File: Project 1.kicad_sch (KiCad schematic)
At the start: 14 parts, among them J1 DB9_Female, J2 Barrel_Jack, P1 RFID-RC522-MODULE, SW1 SW_DPDT_x2, U1 PIC16F1512-ISP, U2 PIC16F1512-ISP, U3 PIC16F1512-ISP, U4 ADG419BN, U5 TM1637, U6 TM1637

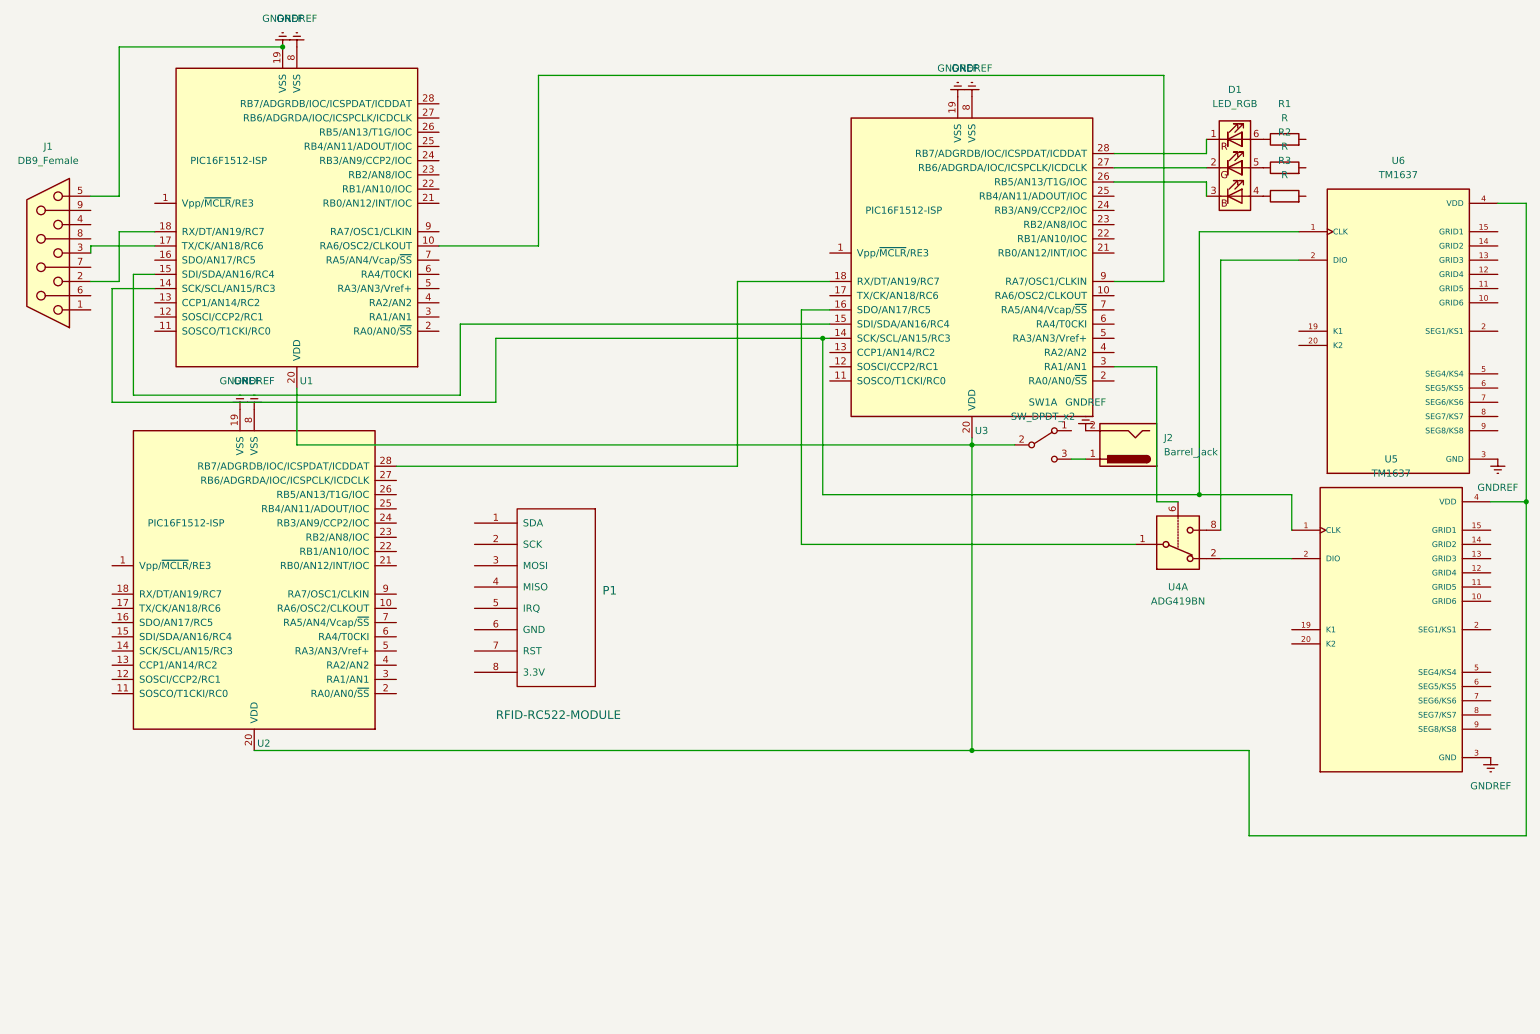
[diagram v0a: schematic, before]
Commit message: Nieuwe tekening begin nieuw schema
Nieuwe tekening begin nieuw schema
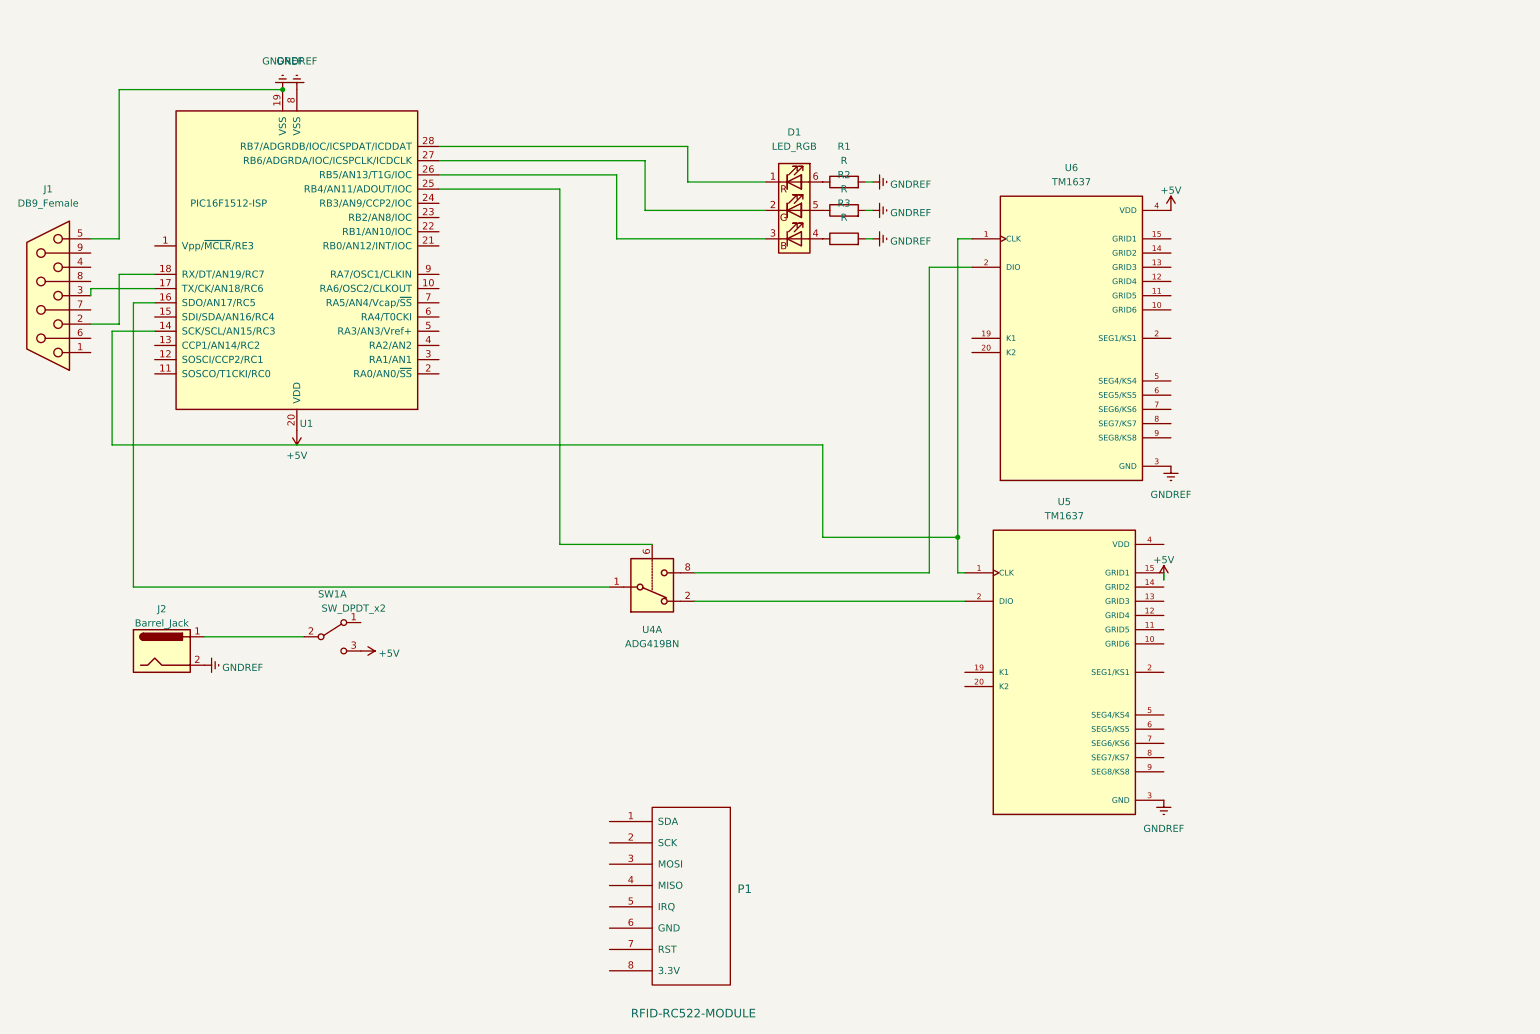
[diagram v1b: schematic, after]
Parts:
- removed U2: PIC16F1512-ISP, Package_DIP:DIP-28_W7.62mm, symbol MCU_Microchip_PIC16:PIC16F1512-ISP
- removed U3: PIC16F1512-ISP, Package_DIP:DIP-28_W7.62mm_Socket, symbol MCU_Microchip_PIC16:PIC16F1512-ISP
- D1: footprint (none) -> LED_SMD:LED_Avago_PLCC6_3x2.8mm
- R1, R2, R3: footprint (none) -> Resistor_SMD:R_0201_0603Metric
- SW1: footprint (none) -> Button_Switch_THT:SW_CuK_JS202011AQN_DPDT_Angled
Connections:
- net GNDREF: now also R1.2, R2.2, R3.2
- net at U6.2 (SEG1/KS1): now also U4.8
- net +5V: now reaches U1.20 (VDD), U6.4 (VDD)
- net +5V: now also SW1.3 (C), U5.15 (GRID1); no longer SW1.2 (B), U5.4 (VDD)
- net at D1.1 (RK): now also U1.28 (RB7/ADGRDB/IOC/ICSPDAT/ICDDAT)
- net at D1.2 (GK): now also U1.27 (RB6/ADGRDA/IOC/ICSPCLK/ICDCLK)
- net at D1.3 (BK): now also U1.26 (RB5/AN13/T1G/IOC)
- net at U5.2 (SEG1/KS1): now also U4.2
- net at J2.1: now also SW1.2 (B); no longer SW1.3 (C)
- net at U4.1: now also U1.16 (SDO/AN17/RC5)
- net at U4.6: now also U1.25 (RB4/AN11/ADOUT/IOC)
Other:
- moved on the sheet: D1, J1, J2, P1, R1, R2, R3, SW1A, U1, U4A, U5, U6

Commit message: ZElfde
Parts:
- P1: footprint Connector_PinHeader_1.27mm:PinHeader_1x08_P1.27mm_Vertical -> Connector_PinSocket_2.54mm:PinSocket_1x08_P2.54mm_Vertical
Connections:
- net at U6.2 (SEG1/KS1): now also U4.8
- net at U5.2 (SEG1/KS1): now also U4.2
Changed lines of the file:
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@@
   (symbol (lib_id "power:+5V") (at 218.44 105.41 0) (unit 1)
     (in_bom yes) (on_board yes) (fields_autoplaced)
-    (property "Reference" "#PWR?" (id 0) (at 218.44 109.22 0)
+    (property "Reference" "#PWR0112" (id 0) (at 218.44 109.22 0)
       (effects (font (size 1.27 1.27)) hide)
     )
@@
   (symbol (lib_id "power:+5V") (at 74.93 118.11 270) (unit 1)
     (in_bom yes) (on_board yes) (fields_autoplaced)
-    (property "Reference" "#PWR?" (id 0) (at 71.12 118.11 0)
+    (property "Reference" "#PWR0104" (id 0) (at 71.12 118.11 0)
       (effects (font (size 1.27 1.27)) hide)
     )
@@
   (symbol (lib_id "power:GNDREF") (at 166.37 34.29 90) (unit 1)
     (in_bom yes) (on_board yes)
-    (property "Reference" "#PWR?" (id 0) (at 172.72 34.29 0)
+    (property "Reference" "#PWR0106" (id 0) (at 172.72 34.29 0)
       (effects (font (size 1.27 1.27)) hide)
     )
@@
   (symbol (lib_id "power:+5V") (at 63.5 78.74 180) (unit 1)
     (in_bom yes) (on_board yes) (fields_autoplaced)
-    (property "Reference" "#PWR?" (id 0) (at 63.5 74.93 0)
+    (property "Reference" "#PWR0105" (id 0) (at 63.5 74.93 0)
       (effects (font (size 1.27 1.27)) hide)
     )
@@
       (effects (font (size 1.524 1.524)) (justify left))
     )
-    (property "Footprint" "Connector_PinHeader_1.27mm:PinHeader_1x08_P1.27mm_Vertical" (id 2) (at 133.35 162.56 0)
+    (property "Footprint" "Connector_PinSocket_2.54mm:PinSocket_1x08_P2.54mm_Vertical" (id 2) (at 133.35 162.56 0)
       (effects (font (size 1.524 1.524)) hide)
     )
@@
   (symbol (lib_id "power:GNDREF") (at 46.99 120.65 90) (unit 1)
     (in_bom yes) (on_board yes) (fields_autoplaced)
-    (property "Reference" "#PWR?" (id 0) (at 53.34 120.65 0)
+    (property "Reference" "#PWR0101" (id 0) (at 53.34 120.65 0)
       (effects (font (size 1.27 1.27)) hide)
     )
@@
   (symbol (lib_id "power:GNDREF") (at 166.37 44.45 90) (unit 1)
     (in_bom yes) (on_board yes) (fields_autoplaced)
-    (property "Reference" "#PWR?" (id 0) (at 172.72 44.45 0)
+    (property "Reference" "#PWR0107" (id 0) (at 172.72 44.45 0)
       (effects (font (size 1.27 1.27)) hide)
     )
@@
   (symbol (lib_id "power:+5V") (at 219.71 39.37 0) (unit 1)
     (in_bom yes) (on_board yes)
-    (property "Reference" "#PWR?" (id 0) (at 219.71 43.18 0)
+    (property "Reference" "#PWR0111" (id 0) (at 219.71 43.18 0)
       (effects (font (size 1.27 1.27)) hide)
     )
@@
   (symbol (lib_id "power:GNDREF") (at 166.37 39.37 90) (unit 1)
     (in_bom yes) (on_board yes)
-    (property "Reference" "#PWR?" (id 0) (at 172.72 39.37 0)
+    (property "Reference" "#PWR0110" (id 0) (at 172.72 39.37 0)
       (effects (font (size 1.27 1.27)) hide)
     )
@@
   )
   (symbol_instances
+    (path "/ba3feac5-d630-4bed-8e14-7db0b42c2f83"
+      (reference "#PWR0101") (unit 1) (value "GNDREF") (footprint "")
+    )
     (path "/c7669069-c13b-42b4-a278-9f48cd76a941"
       (reference "#PWR0102") (unit 1) (value "GNDREF") (footprint "")
@@
       (reference "#PWR0103") (unit 1) (value "GNDREF") (footprint "")
     )
+    (path "/338518ab-5898-4c83-bb50-b440f75027b4"
+      (reference "#PWR0104") (unit 1) (value "+5V") (footprint "")
+    )
+    (path "/78869d40-832b-4402-9c11-4193141d6842"
+      (reference "#PWR0105") (unit 1) (value "+5V") (footprint "")
+    )
+    (path "/6a39bd7f-5728-47af-939f-6a17becf1f25"
+      (reference "#PWR0106") (unit 1) (value "GNDREF") (footprint "")
+    )
+    (path "/cb63e662-501d-4536-84b1-4962a1f99666"
+      (reference "#PWR0107") (unit 1) (value "GNDREF") (footprint "")
+    )
     (path "/d88cfbbf-1cde-4824-a59d-8811cec5ba8c"
       (reference "#PWR0108") (unit 1) (value "GNDREF") (footprint "")
@@
       (reference "#PWR0109") (unit 1) (value "GNDREF") (footprint "")
     )
+    (path "/f606cdc7-a5e0-4feb-bca6-f9655c59631f"
+      (reference "#PWR0110") (unit 1) (value "GNDREF") (footprint "")
+    )
+    (path "/ce0fc0c8-3db8-4941-80cc-972bfb47b4fe"
+      (reference "#PWR0111") (unit 1) (value "+5V") (footprint "")
+    )
     (path "/0a625eb3-7c7b-4204-8a93-2f92b04ba9f2"
-      (reference "#PWR?") (unit 1) (value "+5V") (footprint "")
-    )
-    (path "/338518ab-5898-4c83-bb50-b440f75027b4"
-      (reference "#PWR?") (unit 1) (value "+5V") (footprint "")
-    )
-    (path "/6a39bd7f-5728-47af-939f-6a17becf1f25"
-      (reference "#PWR?") (unit 1) (value "GNDREF") (footprint "")
-    )
-    (path "/78869d40-832b-4402-9c11-4193141d6842"
-      (reference "#PWR?") (unit 1) (value "+5V") (footprint "")
-    )
-    (path "/ba3feac5-d630-4bed-8e14-7db0b42c2f83"
-      (reference "#PWR?") (unit 1) (value "GNDREF") (footprint "")
-    )
-    (path "/cb63e662-501d-4536-84b1-4962a1f99666"
-      (reference "#PWR?") (unit 1) (value "GNDREF") (footprint "")
-    )
-    (path "/ce0fc0c8-3db8-4941-80cc-972bfb47b4fe"
-      (reference "#PWR?") (unit 1) (value "+5V") (footprint "")
-    )
-    (path "/f606cdc7-a5e0-4feb-bca6-f9655c59631f"
-      (reference "#PWR?") (unit 1) (value "GNDREF") (footprint "")
+      (reference "#PWR0112") (unit 1) (value "+5V") (footprint "")
     )
     (path "/2de269c6-be7f-498e-9d9c-81e85907e612"
@@
     )
     (path "/a96f00ba-dda0-463c-ab04-89a38023e407"
-      (reference "P1") (unit 1) (value "RFID-RC522-MODULE") (footprint "Connector_PinHeader_1.27mm:PinHeader_1x08_P1.27mm_Vertical")
+      (reference "P1") (unit 1) (value "RFID-RC522-MODULE") (footprint "Connector_PinSocket_2.54mm:PinSocket_1x08_P2.54mm_Vertical")
     )
     (path "/70e088a3-daab-461b-924b-e4ab67f39b3e"
